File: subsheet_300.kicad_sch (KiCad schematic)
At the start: 37 parts, among them Q11 2N3904, Q6 2N3904, Q7 2N3906, Q8 2N3904, Q9 2N3906, U41 74LS74 DUAL FLIP-FLOPS, Y2 see table, Y3 see table

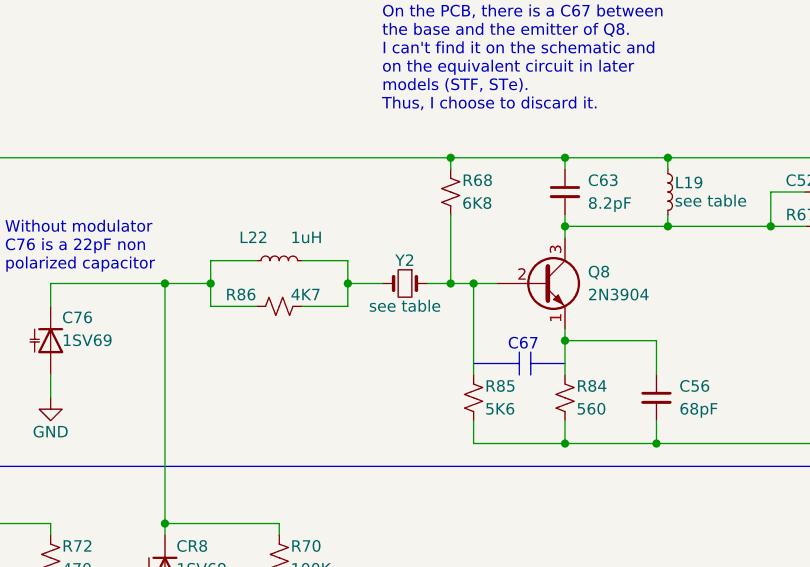
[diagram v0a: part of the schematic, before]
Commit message: pcb session 2023-11-26T22:40:44+01:00 : rework composite circuit after real motherboard -- r140, r141 and q11 invented
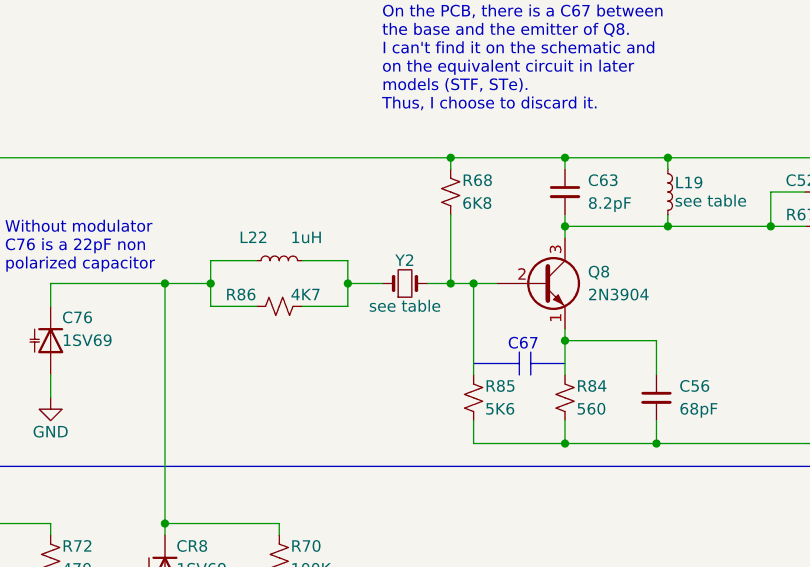
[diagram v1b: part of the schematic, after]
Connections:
- net at Q8.2 (B), R68.1, R85.2: now also Y2.2; no longer Y2.1
- net at L22.2, R86.2: now also Y2.1; no longer Y2.2
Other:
- moved on the sheet: Y2
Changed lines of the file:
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@@
     )
   )
-  (symbol (lib_id "Device:Crystal_Small") (at 99.06 48.26 180) (unit 1)
+  (symbol (lib_id "Device:Crystal_Small") (at 99.06 48.26 0) (unit 1)
     (in_bom yes) (on_board yes) (dnp no)
     (property "Reference" "Y2" (at 99.06 45.72 0)

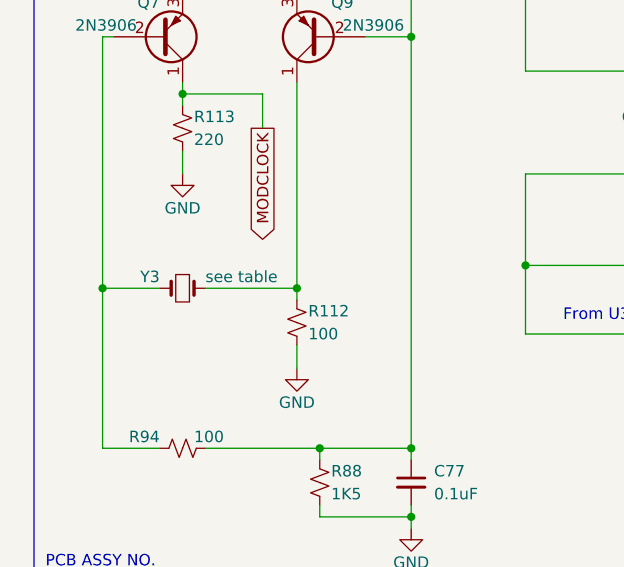
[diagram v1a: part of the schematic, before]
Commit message: pcb session 2023-11-26T23:17:41+01:00
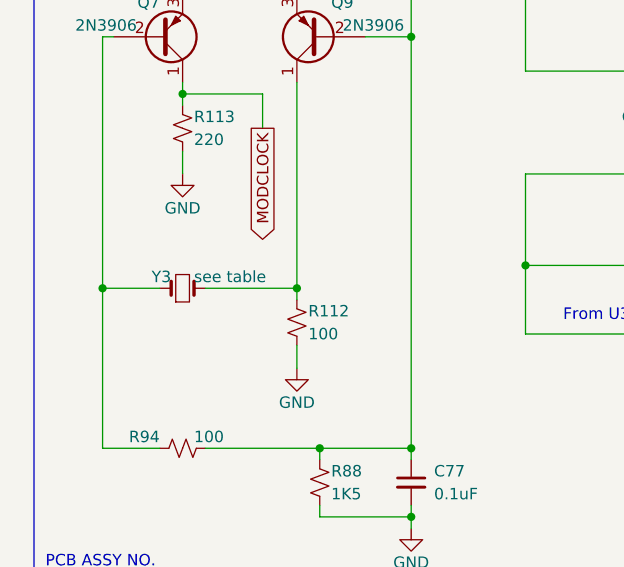
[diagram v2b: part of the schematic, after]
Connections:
- net at Q9.1 (C), R112.2: now also Y3.2; no longer Y3.1
- net at Q7.2 (B), R94.1: now also Y3.1; no longer Y3.2
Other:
- moved on the sheet: Y3
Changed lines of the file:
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@@
     )
   )
-  (symbol (lib_id "Device:Crystal_Small") (at 34.29 116.84 180) (unit 1)
+  (symbol (lib_id "Device:Crystal_Small") (at 34.29 116.84 0) (unit 1)
     (in_bom yes) (on_board yes) (dnp no)
-    (property "Reference" "Y3" (at 31.75 115.57 0)
+    (property "Reference" "Y3" (at 33.02 115.57 0)
+      (effects (font (size 1.27 1.27)) (justify right))
+    )
+    (property "Value" "see table" (at 35.56 115.57 0)
       (effects (font (size 1.27 1.27)) (justify left))
     )
-    (property "Value" "see table" (at 36.83 115.57 0)
-      (effects (font (size 1.27 1.27)) (justify right))
-    )
     (property "Footprint" "Crystal:Crystal_HC50_Horizontal" (at 34.29 116.84 0)
